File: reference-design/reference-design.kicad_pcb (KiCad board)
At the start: 2 copper layers, 104 x 83.9 mm, 31 parts

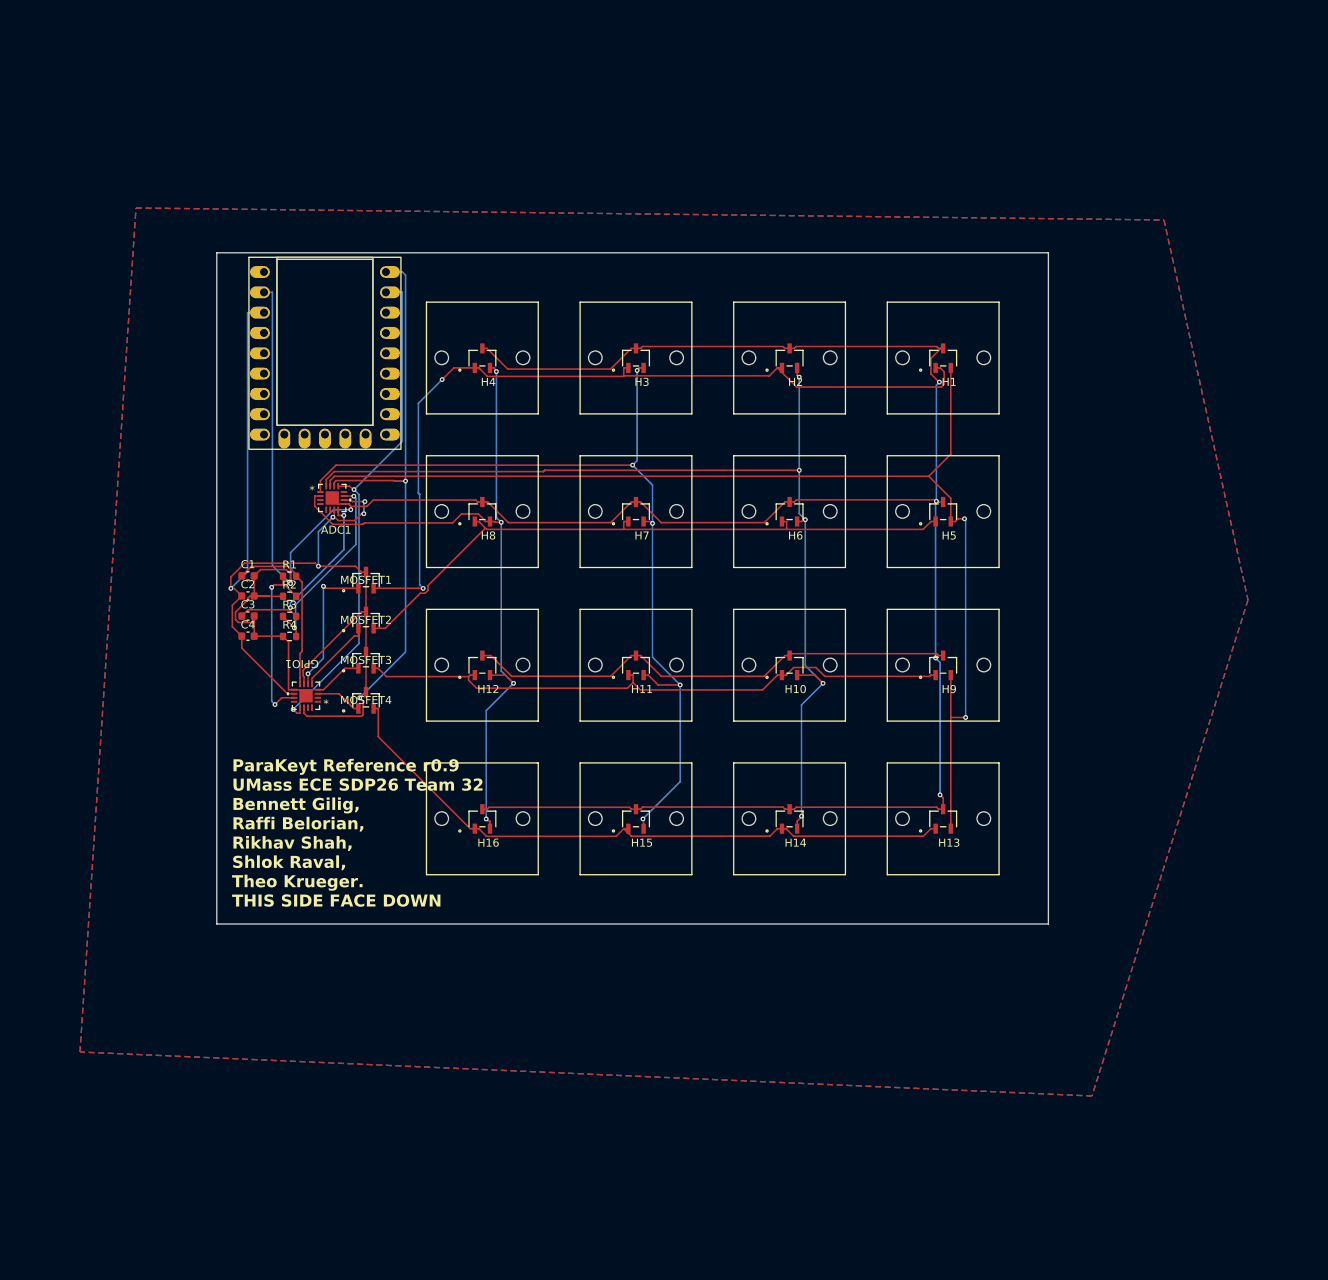
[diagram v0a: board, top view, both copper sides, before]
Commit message: prep for order
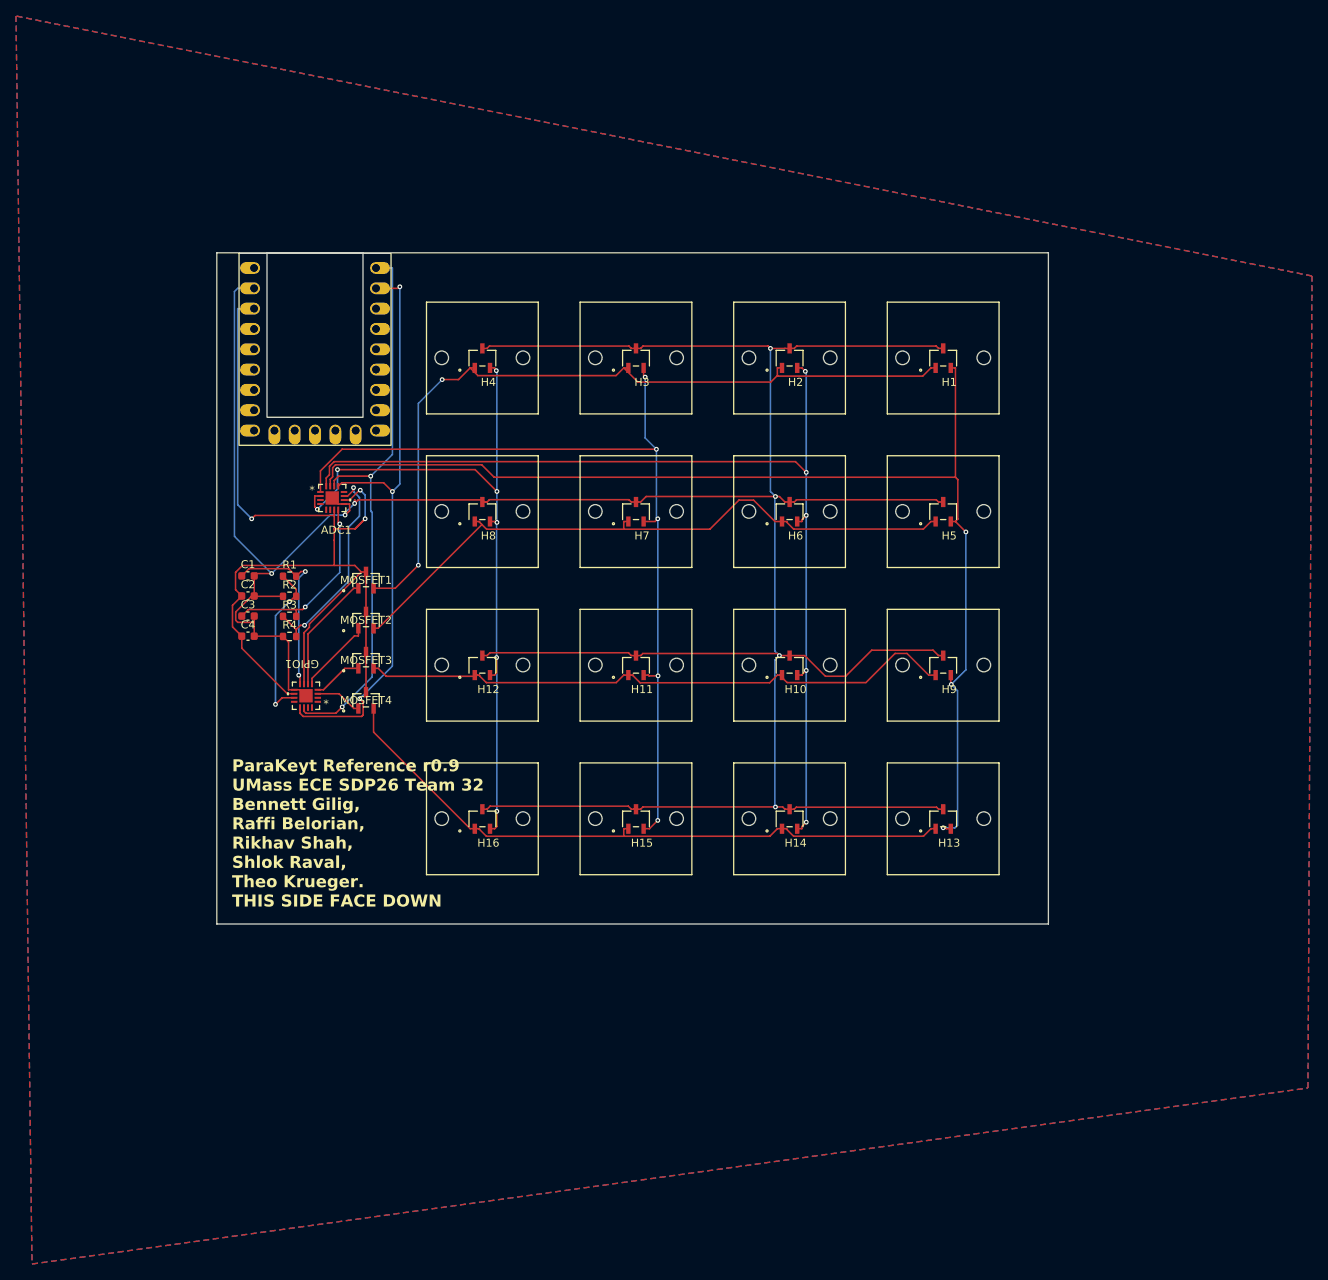
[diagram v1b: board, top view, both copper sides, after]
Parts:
- moved MCU1 1.34 mm to (24.4, 24.2)
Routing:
- net +3.3V: track 119.2 -> 133.4 mm, vias 5 -> 3
- net GND: track 412.4 -> 401.3 mm, vias 6 -> 7
- net i2c0_scl: track 64.5 -> 75.1 mm, vias 2 -> 3
- net i2c0_sda: track 80.7 -> 71.1 mm
- net Net-(H1-VCC): track 104.8 -> 98.5 mm
- net row0: track 18.9 -> 14.9 mm, vias 2 -> 0
- net Net-(ADC1-ADDR): track 24.2 -> 27.4 mm
- net Net-(GPIO1-ADDR): track 22.4 -> 20.6 mm
- net Net-(GPIO1-DECAP): track 21.8 -> 23.4 mm, vias 0 -> 2
- net col2: track 110.5 -> 109.1 mm
- net Net-(H5-VCC): track 81.1 -> 81.9 mm
- net col3: track 91.7 -> 92.4 mm, vias 4 -> 7
- net col0: track 145.0 -> 145.4 mm, vias 2 -> 3
